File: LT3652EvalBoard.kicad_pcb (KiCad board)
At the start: 2 copper layers, 55.2 x 50.3 mm, 42 parts, among them U1 LT3652

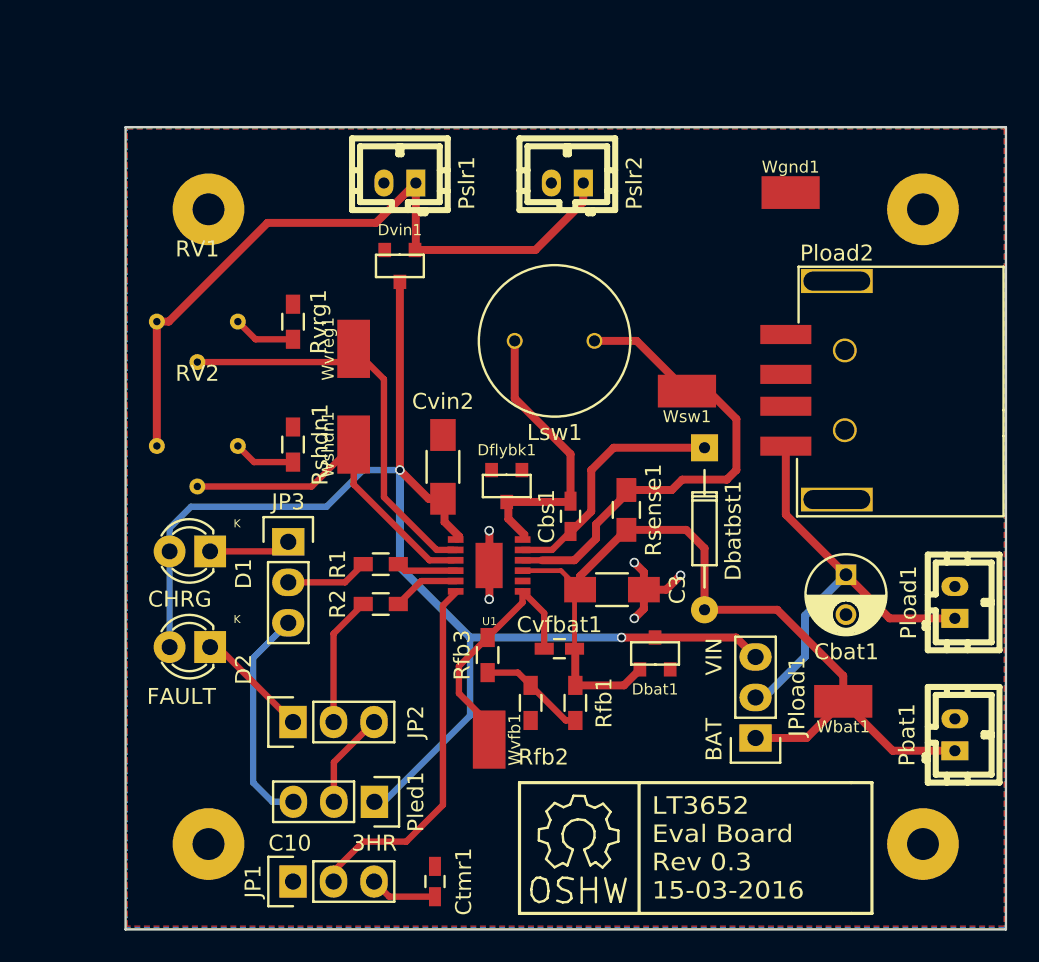
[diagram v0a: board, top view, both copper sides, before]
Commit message: Upload of Rev 0.5
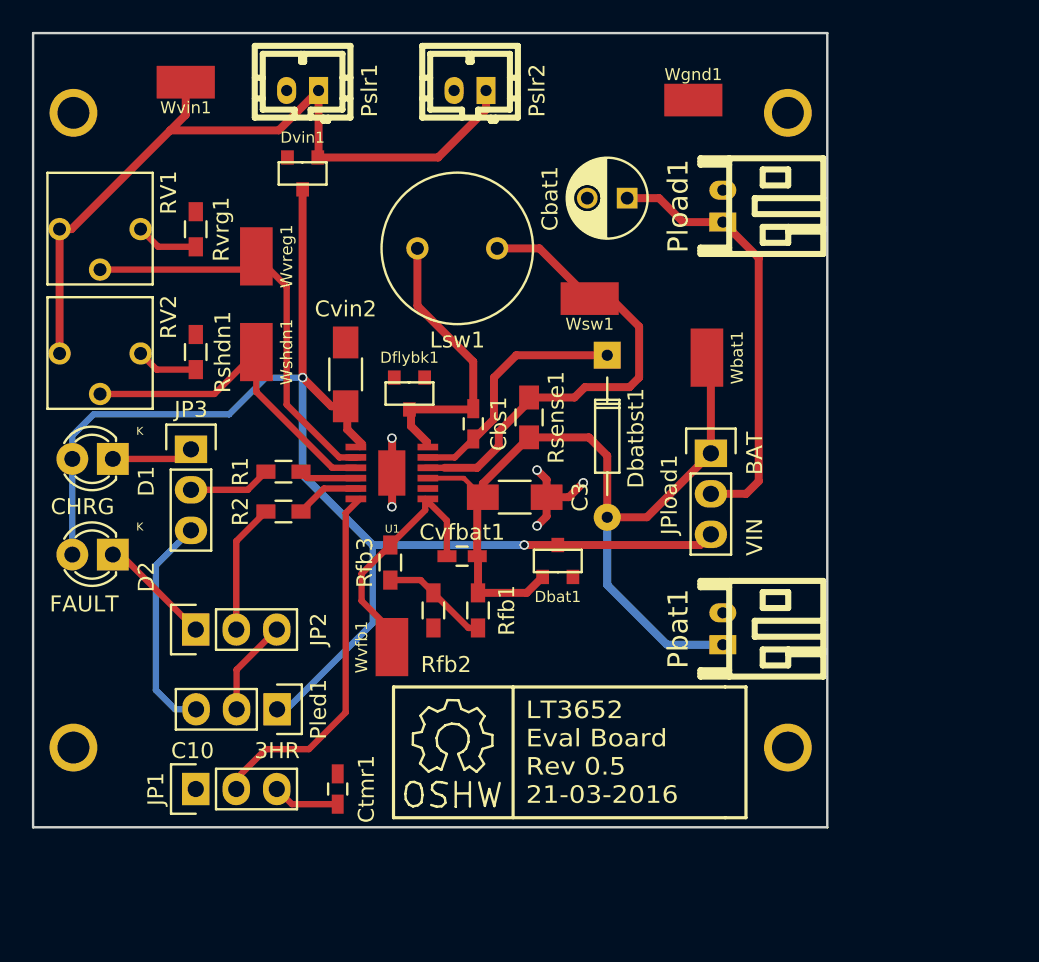
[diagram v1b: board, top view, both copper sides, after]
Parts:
- removed the ? at (143.9, 95.8)
- removed Pload2: USB_A, ms_connectors:WURTH_ELEKTRONIK_629104151021
- added REF**: MHH-20_ABS_Plastic_Box, ms_enclosures:MHH-20_ABS_Plastic_Box_Holes_Only, F.Cu at (135.4, 89.7)
- added Wvin1: TEST_1P, ms_pcb_test_points:HARWIN_S1751-46, F.Cu at (119.6, 68.4)
- Pbat1, Pload1: footprint w_conn_jst-ph:b2b-ph-kl -> w_conn_jst-ph:s2b-ph-kl
- U1: footprint ms_lt3652:LT3652MSE -> ms_lt3652:LT3652MSE_HandSoldering
- moved Pload1 28.8 mm to (153.3, 76.2)
- moved Cbat1 27.3 mm to (147.3, 75.7), turned to 180 degrees
- moved Wbat1 23.2 mm to (152.3, 85.7), turned to 90 degrees
- moved JPload1 18.1 mm to (152.6, 91.7), turned to 0 degrees
- moved Pbat1 16.0 mm to (153.3, 102.7)
- moved ? 9.92 mm to (136.4, 109.7)
- moved C3 8.42 mm to (140.3, 94.5)
- moved R1 8.42 mm to (125.8, 92.8)
- moved R2 8.42 mm to (125.8, 95.3)
- moved Cbs1 8.42 mm to (137.7, 89.8)
- moved Dvin1 8.42 mm to (127.0, 74.2)
- moved JP3 8.42 mm to (120.0, 91.5)
- moved Lsw1 8.42 mm to (136.7, 78.8)
- moved Pled1 8.42 mm to (125.4, 107.8)
- moved Pslr1 8.42 mm to (127.0, 69.0)
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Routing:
- net Net-(Dvin1-Pad3): track 44.9 -> 48.3 mm
- net /VIN: track 88.6 -> 91.6 mm
- net /BAT: track 56.7 -> 57.8 mm
- net Net-(Cbat1-Pad1): track 28.0 -> 27.1 mm
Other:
- board size 55.2 x 50.3 mm -> 49.8 x 49.8 mm
- board text added: "LT3652 Eval Board Rev 0.5 21-03-2016"
- board text removed: "LT3652 Eval Board Rev 0.3 15-03-2016"
